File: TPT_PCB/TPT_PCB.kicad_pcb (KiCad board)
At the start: 2 copper layers, 79.8 x 74.2 mm, 55 parts, among them J1 Conn_01x04, J2 Conn_01x04, J3 Conn_01x04, J4 Conn_01x04, J5 Conn_01x04, J6 SWD, J7 Power, J8 Conn_01x06, SW1 SW_Push, U1 TCA9548APWR, U2 RT9013, U3 STM32F103RCT6, Y1 8MHz, Y2 32.768kHz

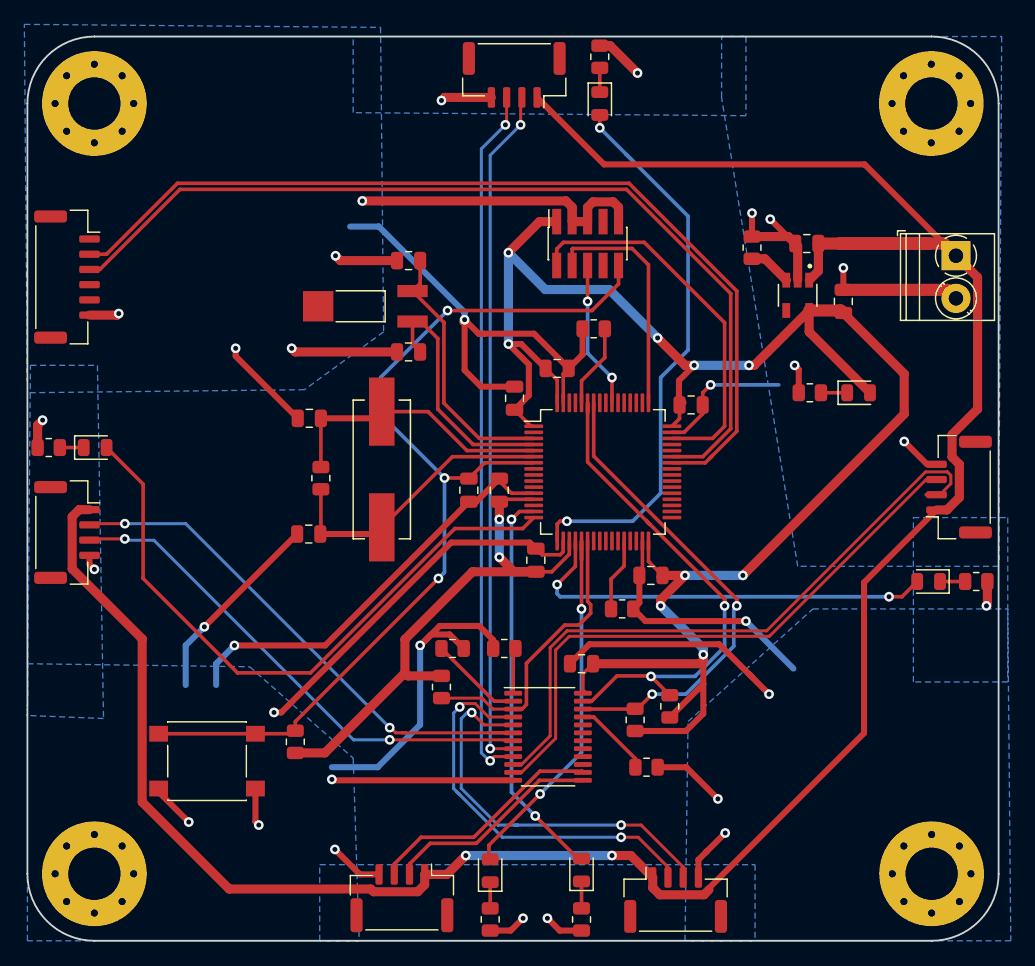
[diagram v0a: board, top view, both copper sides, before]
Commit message: re-layout and generate gbr file
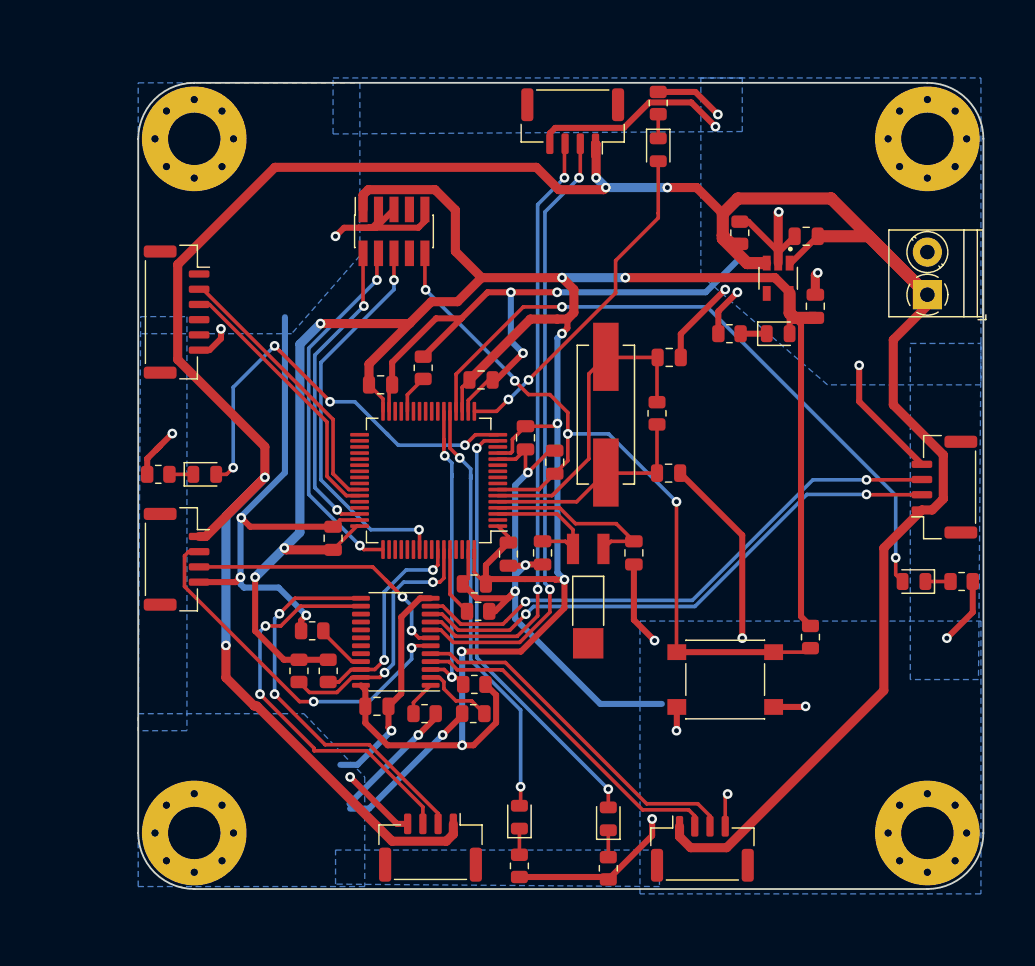
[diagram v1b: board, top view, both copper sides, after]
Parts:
- moved R7 43.2 mm to (179.4, 105.9), turned to 270 degrees
- moved SW1 43.1 mm to (172.4, 109.4)
- moved C3 33.0 mm to (167.8, 83.0), turned to 0 degrees
- moved C11 31.4 mm to (140.2, 97.8), turned to 90 degrees
- moved R2 30.6 mm to (137.4, 108.7), turned to 270 degrees
- moved Y2 30.0 mm to (161.2, 102.5), turned to 90 degrees
- moved C2 29.8 mm to (167.8, 92.5), turned to 0 degrees
- moved R3 29.6 mm to (138.5, 105.4), turned to 180 degrees
- moved R8 28.1 mm to (166.8, 87.5), turned to 90 degrees
- moved C12 27.2 mm to (144.1, 85.2), turned to 0 degrees
- moved C4 26.4 mm to (157.4, 99.0), turned to 270 degrees
- moved R10 25.7 mm to (147.6, 83.8), turned to 90 degrees
- moved R6 25.5 mm to (139.8, 108.7), turned to 270 degrees
- moved R9 25.1 mm to (152.1, 103.8), turned to 0 degrees
- moved C5 24.8 mm to (164.9, 99.0), turned to 270 degrees
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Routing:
- net /UART1_TX: track 77.5 -> 22.6 mm
- net /UART1_RX: track 75.8 -> 22.3 mm
- net +3V3: track 198.7 -> 240.6 mm, vias 11 -> 10
- net Master_SCL: track 39.6 -> 17.5 mm
- net GND: track 347.8 -> 325.8 mm, vias 31 -> 30
- net /SWO: track 12.1 -> 33.3 mm
- net Master_SDA: track 42.0 -> 21.9 mm
- net /Left_LED: track 35.1 -> 55.1 mm
- net /Rear_LED: track 47.2 -> 27.9 mm
- net +5V: track 210.6 -> 229.7 mm, vias 2 -> 5
- net /Right_SCL: track 42.4 -> 23.5 mm
- net /Right_LED: track 52.6 -> 35.9 mm, vias 0 -> 4
- net /NRST: track 79.7 -> 64.3 mm, vias 3 -> 4
- net /Upward_SDA: track 17.9 -> 32.3 mm, vias 0 -> 2
- net /Right_SDA: track 45.0 -> 31.3 mm
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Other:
- board size 79.8 x 74.2 mm -> 69.4 x 66.2 mm
